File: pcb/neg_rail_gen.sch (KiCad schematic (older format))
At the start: 25 parts, among them U5 LM2596S-ADJ

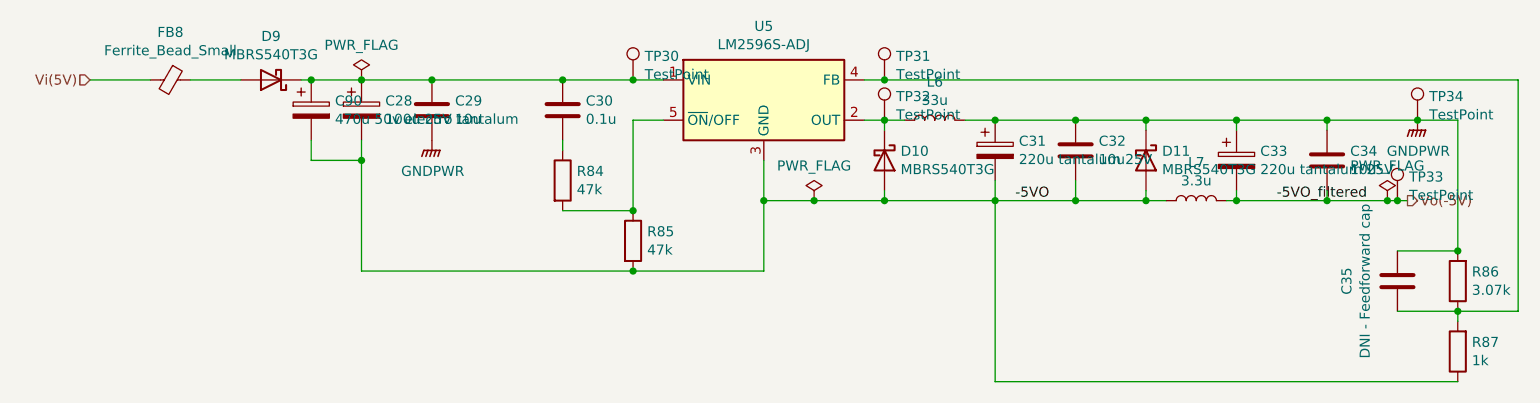
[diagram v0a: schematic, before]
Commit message: layout progress
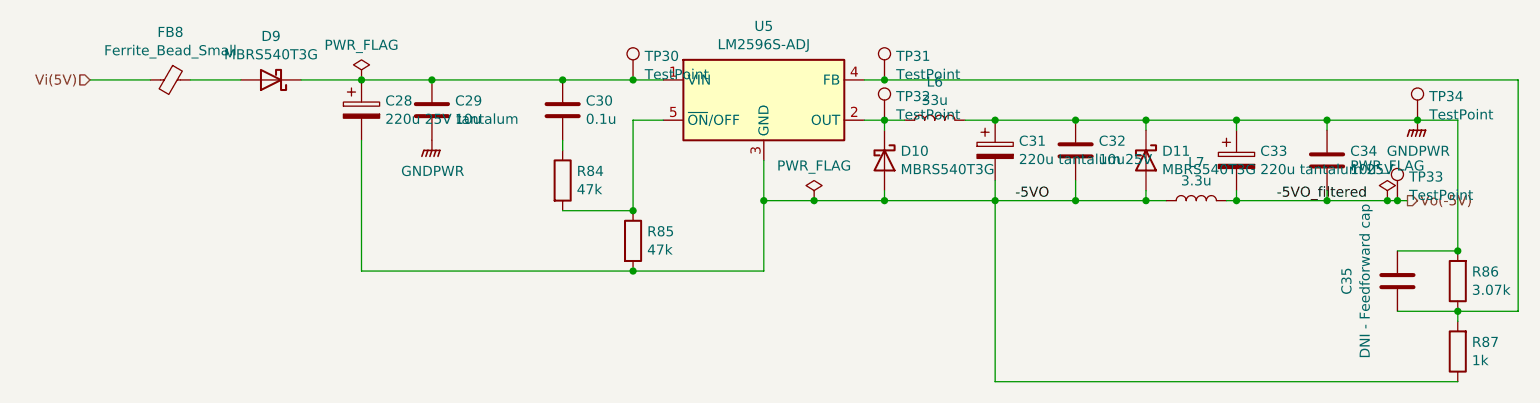
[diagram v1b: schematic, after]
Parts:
- removed C90: 470u 50v electro, Capacitor_THT:C_Radial_D10.0mm_H20.0mm_P5.00mm, symbol Device:CP
- C28: value 100u 25V tantalum -> 220u 25V tantalum
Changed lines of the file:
@@
 P 3800 3550
 F 0 "C28" H 3918 3596 50  0000 L CNN
-F 1 "100u 25V tantalum" H 3918 3505 50  0000 L CNN
+F 1 "220u 25V tantalum" H 3918 3505 50  0000 L CNN
 F 2 "Capacitor_Tantalum_SMD:CP_EIA-7343-20_Kemet-V_Pad2.25x2.55mm_HandSolder" H 3838 3400 50  0001 C CNN
 F 3 "~" H 3800 3550 50  0001 C CNN
@@
 Wire Wire Line
 	4800 3700 4800 3750
-Wire Wire Line
-	3500 3400 3550 3400
 Wire Wire Line
 	4150 3400 4800 3400
@@
 	2950 3400 3200 3400
 Wire Wire Line
-	3800 3700 3800 3800
-Wire Wire Line
 	3800 4350 5150 4350
 Connection ~ 5150 4350
@@
 	0    1    1    0
 $EndComp
-$Comp
-L Device:CP C90
-U 1 1 5FBC18F7
-P 3550 3550
-F 0 "C90" H 3668 3596 50  0000 L CNN
-F 1 "470u 50v electro" H 3668 3505 50  0000 L CNN
-F 2 "Capacitor_THT:C_Radial_D10.0mm_H20.0mm_P5.00mm" H 3588 3400 50  0001 C CNN
-F 3 "~" H 3550 3550 50  0001 C CNN
-	1    3550 3550
-	1    0    0    -1
-$EndComp
-Connection ~ 3550 3400
-Wire Wire Line
-	3550 3400 3800 3400
-Wire Wire Line
-	3550 3700 3550 3800
-Wire Wire Line
-	3550 3800 3800 3800
-Connection ~ 3800 3800
-Wire Wire Line
-	3800 3800 3800 4350
 Text Label 7050 4000 0    50   ~ 0
 -5VO
 Text Label 8350 4000 0    50   ~ 0
 -5VO_filtered
+Wire Wire Line
+	3500 3400 3800 3400
+Wire Wire Line
+	3800 3700 3800 4350
 $EndSCHEMATC
